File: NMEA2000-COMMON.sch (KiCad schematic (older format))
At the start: 65 parts, among them J2 CAN, SW1 PRG, SW2 INSTANCE, SW3 BUS, U1 MCP2551-I-P, U101 74LS165, U2 TMR-2-2411, U3 74HCT595, U4 74HCT595, U5 Teensy_4.0

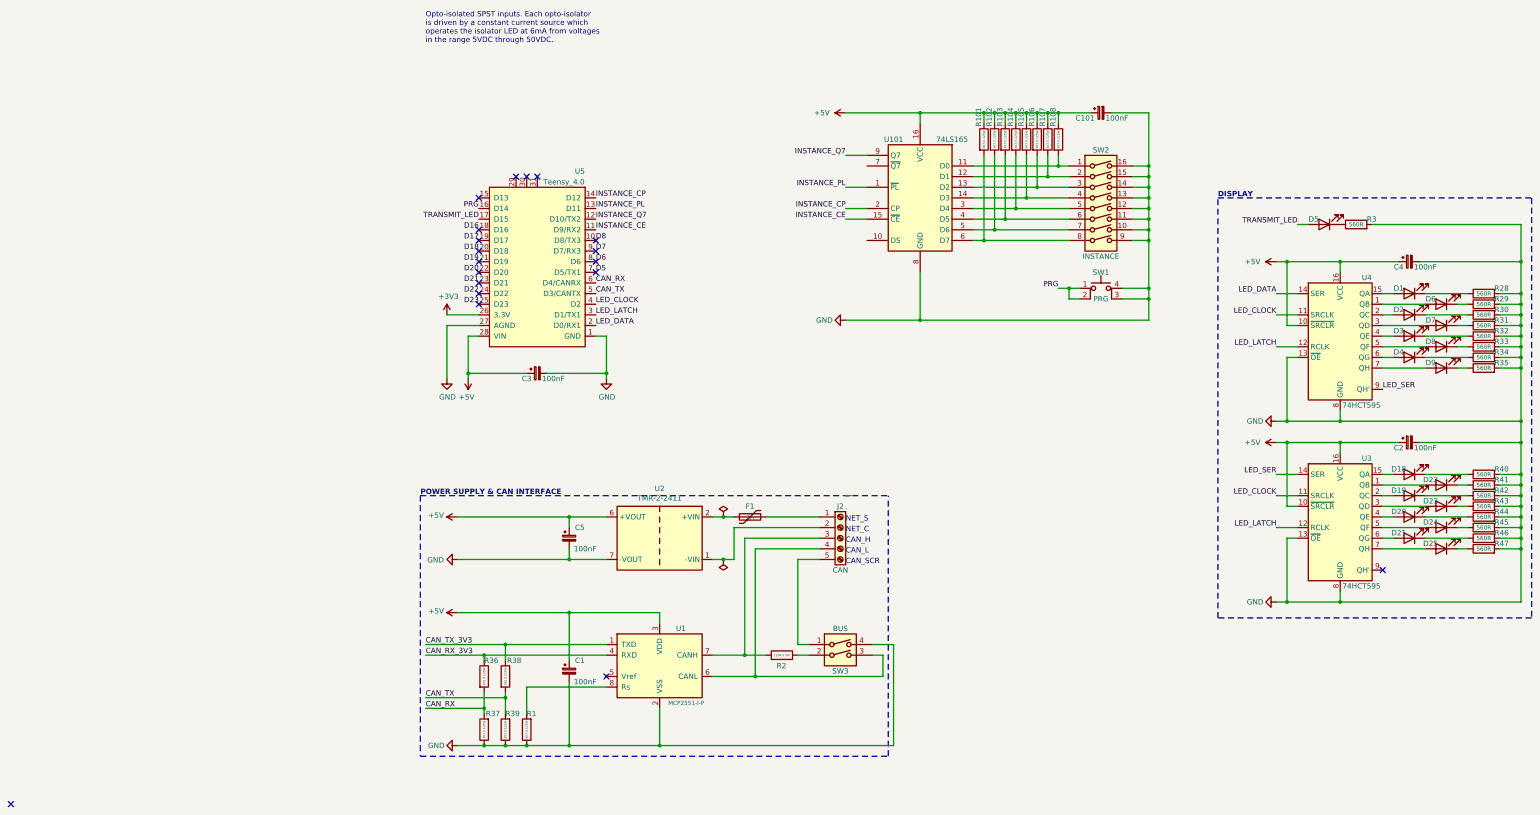
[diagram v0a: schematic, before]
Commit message: Tidy up
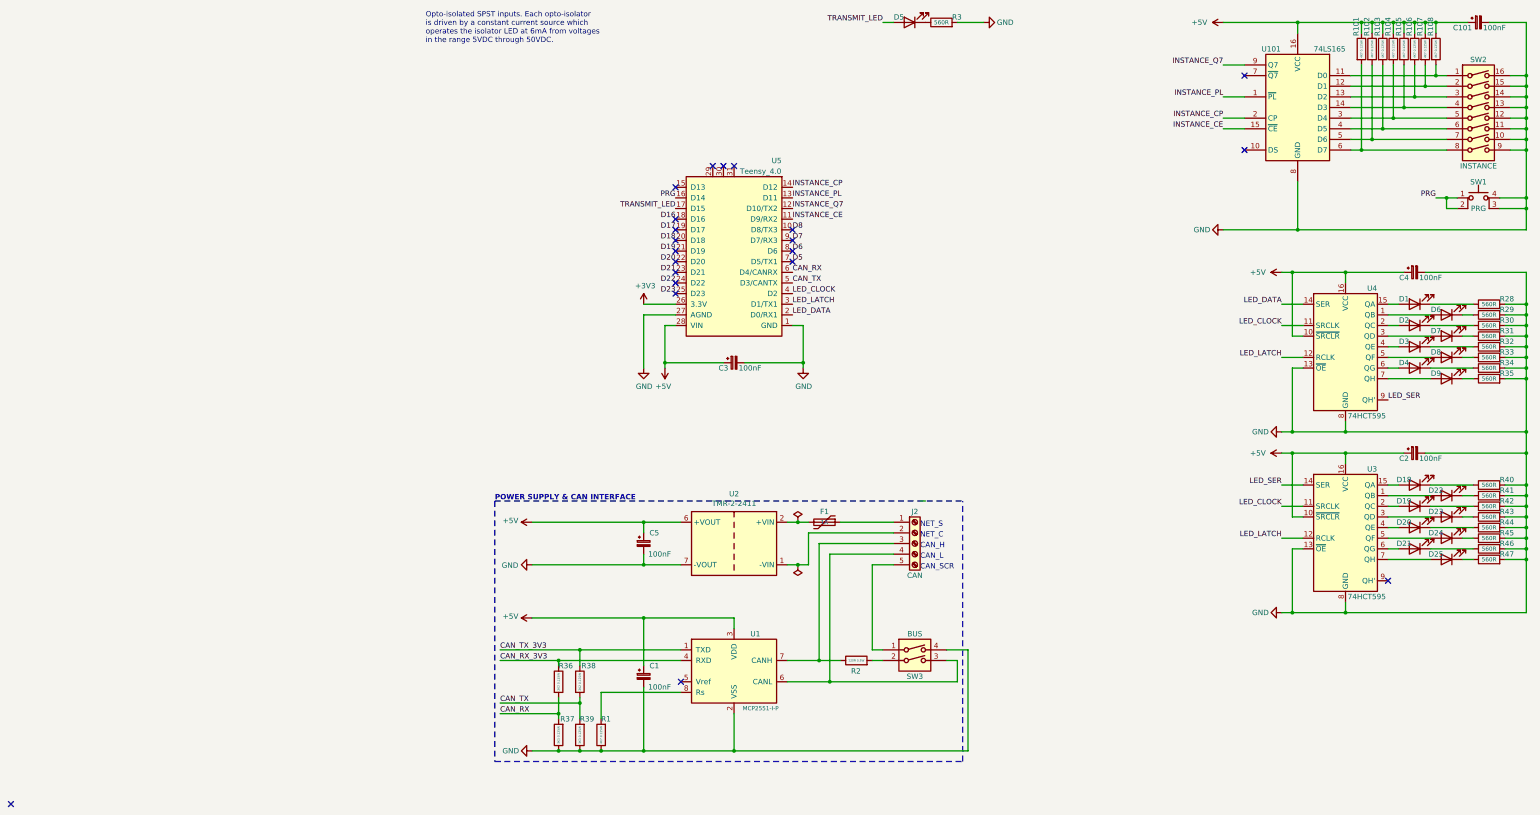
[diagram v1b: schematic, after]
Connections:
- no-connect marks 19 -> 21
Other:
- note removed: "DISPLAY"
- moved on the sheet: C1, C101, C2, C3, C4, C5, D1, D18, D19, D2, D20, D21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
